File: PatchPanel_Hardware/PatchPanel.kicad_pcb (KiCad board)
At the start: 2 copper layers, 172.1 x 75.6 mm, 89 parts, among them Q1 Q_PMOS_DGS, Q10 Q_NMOS_DGS, Q11 Q_NMOS_DGS, Q12 Q_NMOS_DGS, Q13 Q_NMOS_DGS, Q14 Q_NMOS_DGS, Q15 Q_NMOS_DGS, Q16 Q_NMOS_DGS, Q17 Q_PMOS_DGS, Q18 Q_PMOS_DGS, Q19 Q_PMOS_DGS, Q2 Q_PMOS_DGS, Q20 Q_PMOS_DGS, Q21 Q_PMOS_DGS, Q22 Q_PMOS_DGS, Q23 Q_PMOS_DGS, Q24 Q_PMOS_DGS, Q25 Q_NMOS_DGS, Q26 Q_NMOS_DGS, Q27 Q_NMOS_DGS, Q28 Q_NMOS_DGS, Q29 Q_NMOS_DGS, Q3 Q_PMOS_DGS, Q30 Q_NMOS_DGS, Q31 Q_NMOS_DGS, Q32 Q_NMOS_DGS, Q4 Q_PMOS_DGS, Q5 Q_PMOS_DGS, Q6 Q_PMOS_DGS, Q7 Q_PMOS_DGS, Q8 Q_PMOS_DGS, Q9 Q_NMOS_DGS

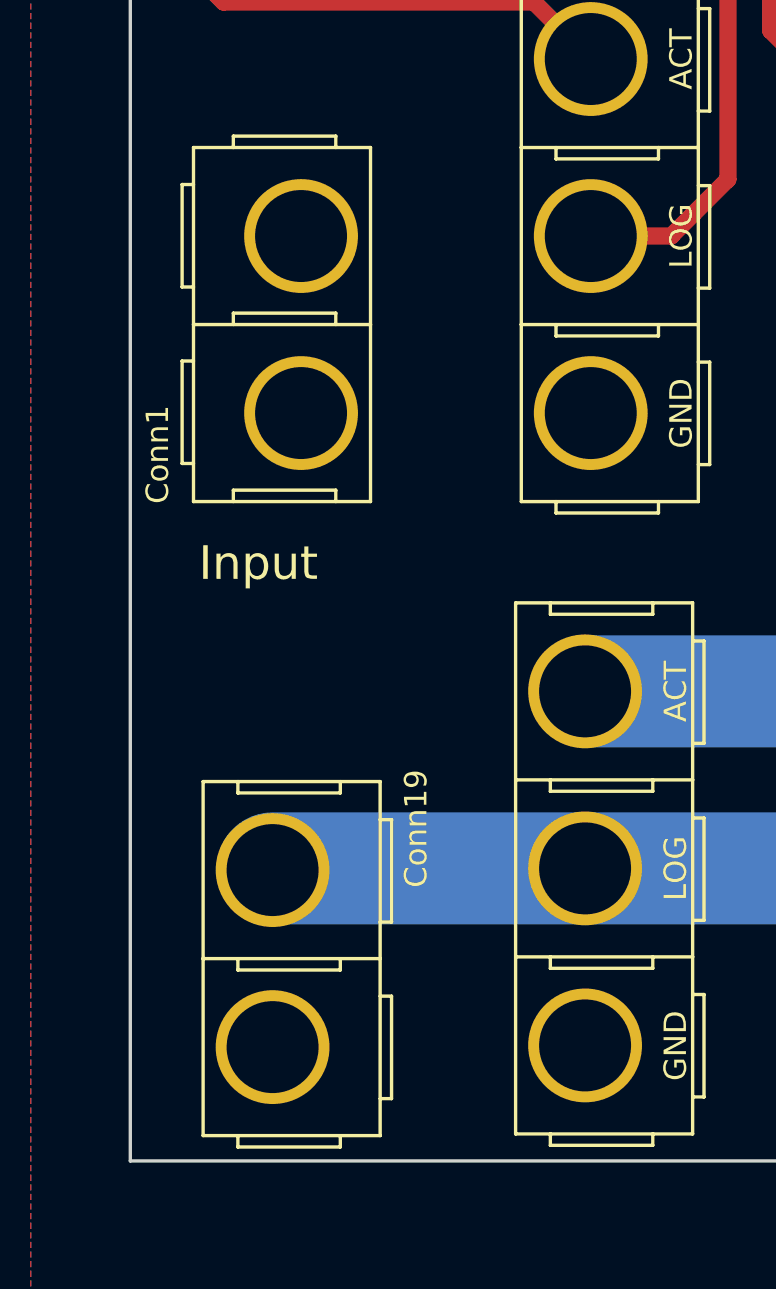
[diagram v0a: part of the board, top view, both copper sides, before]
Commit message: before review
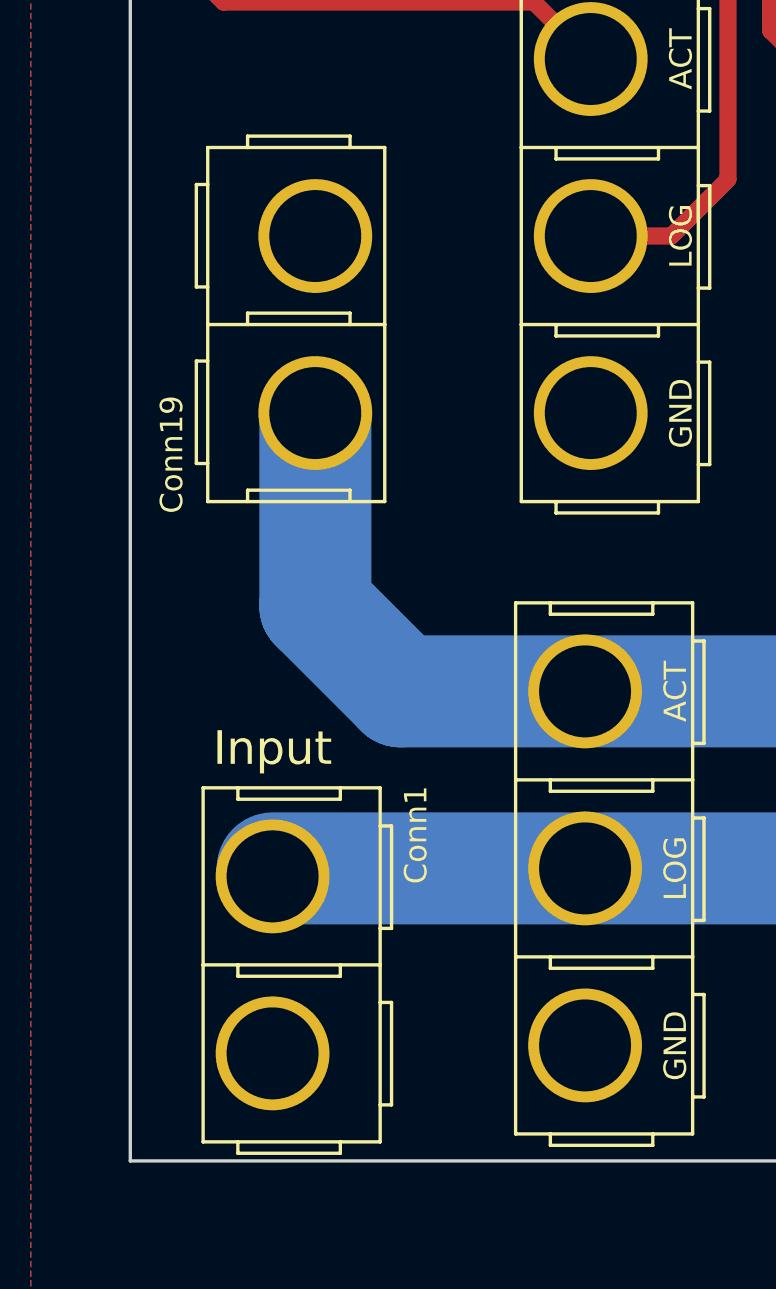
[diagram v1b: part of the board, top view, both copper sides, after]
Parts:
- moved Conn1 45.2 mm to (46.1, 109.6), turned to 90 degrees
- moved Conn19 44.8 mm to (38.4, 65.3), turned to 270 degrees
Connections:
- Conn1 pad 2: (no net) -> /Vlog
- Conn19 pad 2: /Vlog -> /Vact
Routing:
- net /Vact: track 411.0 -> 433.3 mm
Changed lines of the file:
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@@
     (thickness 1.6)
     (drawings 6)
-    (tracks 425)
+    (tracks 428)
     (zones 0)
     (modules 89)
@@
   )
   (module MRDT_Connectors:Anderson_2_Vertical_Sidy_by_Side (layer F.Cu)
-    (at 37.745 65.265 270)
-    (fp_text reference Conn1 (at 13.7 1.6 270) (layer F.SilkS)
+    (at 46.075 109.64 90)
+    (fp_text reference Conn1 (at 13.7 1.6 90) (layer F.SilkS)
       (effects (font (size 1 1) (thickness 0.15)))
     )
-    (fp_text value AndersonPP (at 8.2 -9.2 90) (layer F.Fab) hide
+    (fp_text value AndersonPP (at 8.2 -9.2 270) (layer F.Fab) hide
       (effects (font (size 1 1) (thickness 0.15)))
     )
@@
     (fp_line (start 7.9 -7.9) (end 0 -7.9) (layer F.SilkS) (width 0.15))
     (fp_line (start 7.9 0) (end 0 0) (layer F.SilkS) (width 0.15))
-    (pad 2 thru_hole circle (at 11.85 -4.8 180) (size 5.08 5.08) (drill 4.104006) (layers *.Cu *.Mask))
-    (pad 1 thru_hole circle (at 3.95 -4.8 180) (size 5.08 5.08) (drill 4.104006) (layers *.Cu *.Mask)
+    (pad 2 thru_hole circle (at 11.85 -4.8) (size 5.08 5.08) (drill 4.104006) (layers *.Cu *.Mask)
+      (net 20 /Vlog))
+    (pad 1 thru_hole circle (at 3.95 -4.8) (size 5.08 5.08) (drill 4.104006) (layers *.Cu *.Mask)
       (net 19 GND))
     (model "${MRDT_KICAD_LIBRARIES}/3D Files/MRDT_Connctors/Anderson_2_Vertcal_Side_by_Side.stp"
@@
   )
   (module MRDT_Connectors:Anderson_2_Vertical_Sidy_by_Side (layer F.Cu)
-    (at 46.075 109.36 90)
-    (fp_text reference Conn19 (at 13.7 1.6 90) (layer F.SilkS)
+    (at 38.38 65.265 270)
+    (fp_text reference Conn19 (at 13.7 1.6 270) (layer F.SilkS)
       (effects (font (size 1 1) (thickness 0.15)))
     )
-    (fp_text value AndersonPP (at 8.2 -9.2 270) (layer F.Fab) hide
+    (fp_text value AndersonPP (at 8.2 -9.2 90) (layer F.Fab) hide
       (effects (font (size 1 1) (thickness 0.15)))
     )
@@
     (fp_line (start 15.8 0) (end 15.8 -7.9) (layer F.SilkS) (width 0.15))
     (fp_line (start 15.292 -6.35) (end 15.292 -1.778) (layer F.SilkS) (width 0.15))
-    (pad 1 thru_hole circle (at 3.95 -4.8) (size 5.08 5.08) (drill 4.104006) (layers *.Cu *.Mask)
+    (pad 1 thru_hole circle (at 3.95 -4.8 180) (size 5.08 5.08) (drill 4.104006) (layers *.Cu *.Mask)
       (net 19 GND))
-    (pad 2 thru_hole circle (at 11.85 -4.8) (size 5.08 5.08) (drill 4.104006) (layers *.Cu *.Mask)
-      (net 20 /Vlog))
+    (pad 2 thru_hole circle (at 11.85 -4.8 180) (size 5.08 5.08) (drill 4.104006) (layers *.Cu *.Mask)
+      (net 21 /Vact))
     (model "${MRDT_KICAD_LIBRARIES}/3D Files/MRDT_Connctors/Anderson_2_Vertcal_Side_by_Side.stp"
       (offset (xyz 15.87499976158142 6.984999895095826 0))
@@
     )
   )
-  (gr_text Input (at 40.64 83.82) (layer F.SilkS)
+  (gr_text Input (at 41.275 92.075) (layer F.SilkS)
     (effects (font (size 1.5 1.5) (thickness 0.3)))
   )
@@
   (segment (start 145.3134 55.9816) (end 144.78 56.515) (width 0.762) (layer F.Cu) (net 21))
   (segment (start 145.3134 52.5272) (end 145.3134 55.9816) (width 0.762) (layer F.Cu) (net 21))
+  (segment (start 55.2196 89.535) (end 46.99 89.535) (width 5) (layer B.Cu) (net 21))
+  (segment (start 43.18 85.725) (end 43.18 77.115) (width 5) (layer B.Cu) (net 21))
+  (segment (start 46.99 89.535) (end 43.18 85.725) (width 5) (layer B.Cu) (net 21))
   (segment (start 151.3446 37.3634) (end 154.0764 37.3634) (width 0.381) (layer F.Cu) (net 22))
   (segment (start 151.384 40.1574) (end 154.1158 40.1574) (width 0.381) (layer F.Cu) (net 23))
